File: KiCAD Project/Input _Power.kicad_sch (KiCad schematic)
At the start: 11 parts, among them J1 PJ-102B, Q1 BUK6D120-60PX

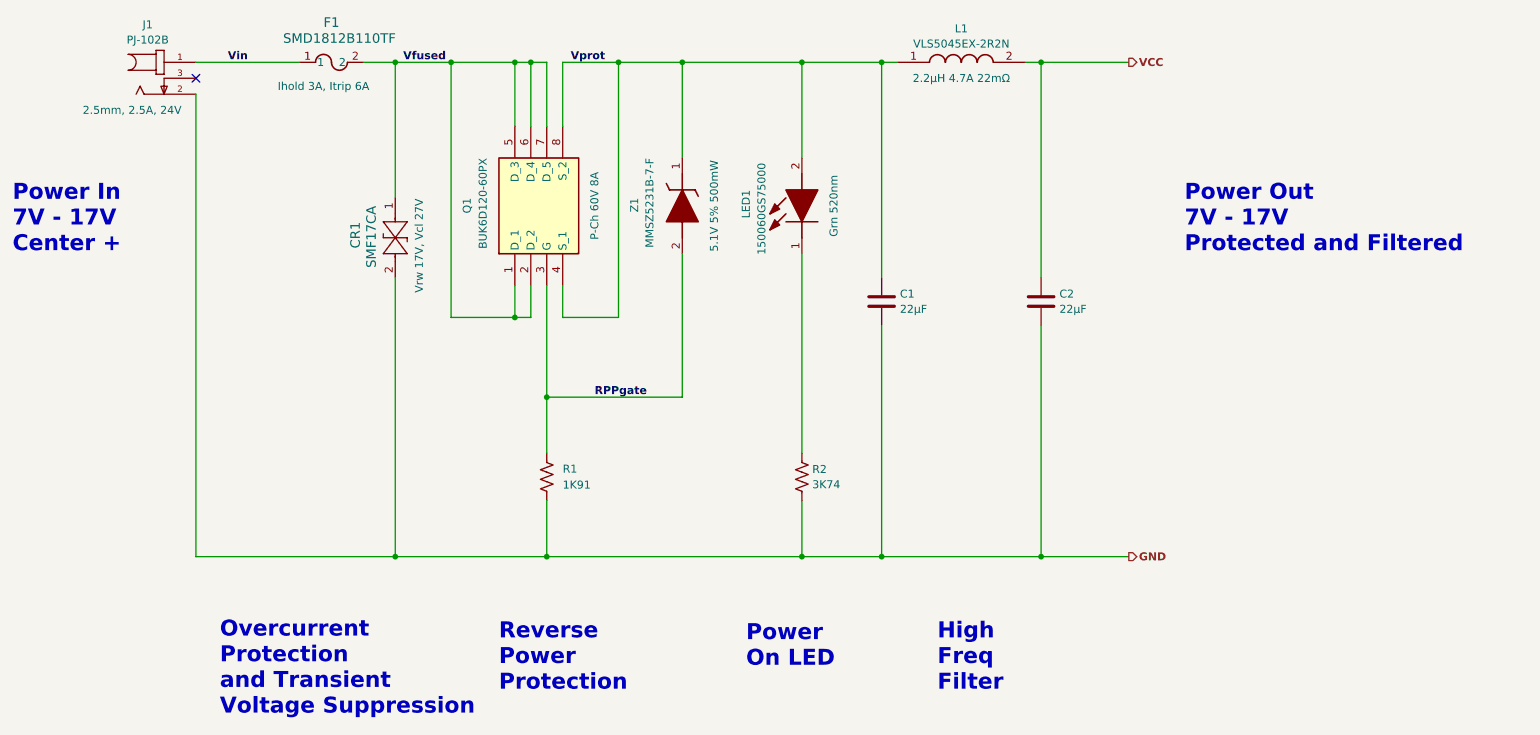
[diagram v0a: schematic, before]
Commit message: V1.0.0.0
Final version 1, sent for fabrication.
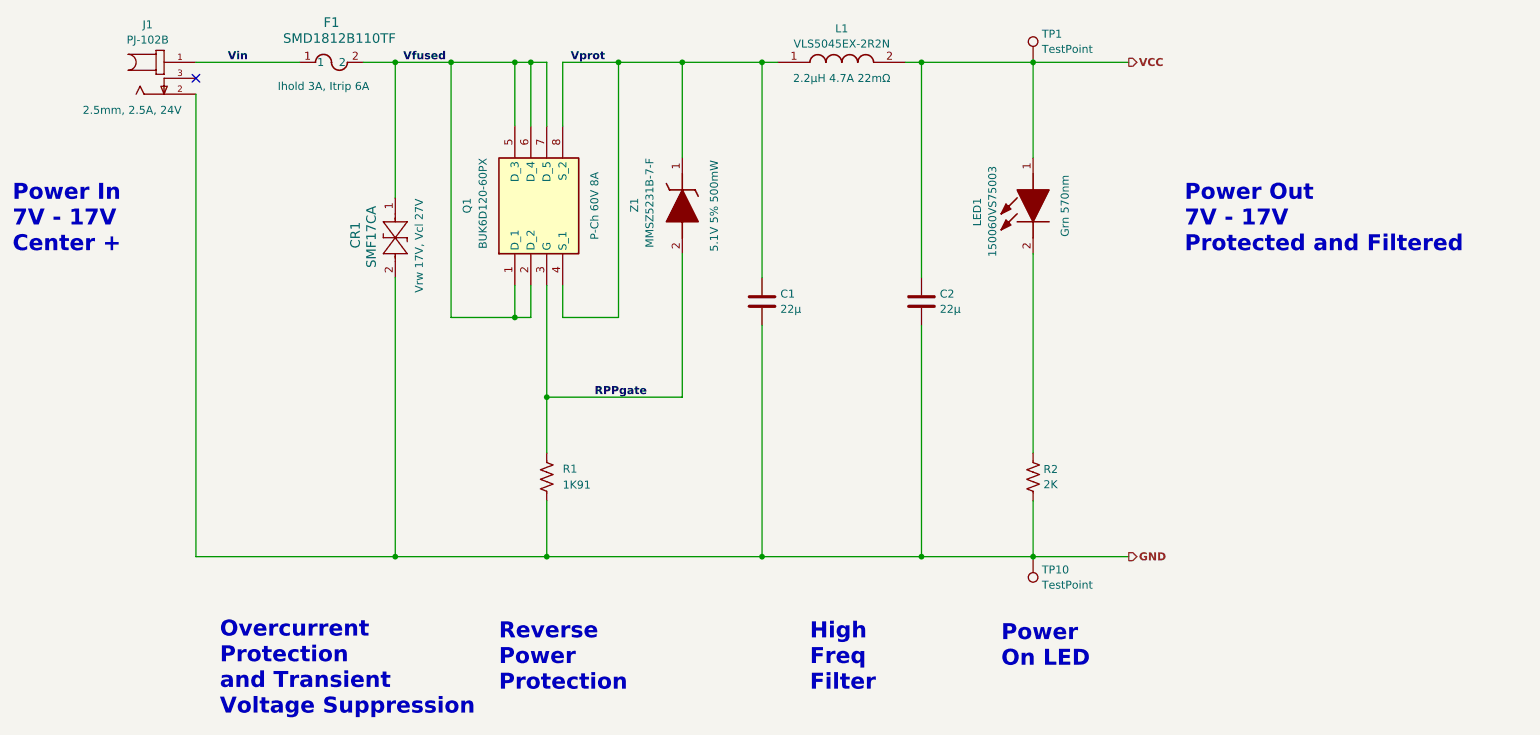
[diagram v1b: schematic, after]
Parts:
- removed LED1: 150060GS75000, LEDC1608X80N, symbol 1016:150060GS75000
- added LED1: 150060VS75003, 1016:LEDC1608X80N, symbol 1016:150060VS75003
- added TP1, TP10: TestPoint, TestPoint:TestPoint_THTPad_D1.0mm_Drill0.5mm, symbol Connector:TestPoint
- C1, C2: value 22µF -> 22µ; LCSC Part Number (none) -> C602037; Spec 22µF 25V -> 22µ 25V
- CR1: Manufacturer_Part_Number C3719828 -> SMF17CA
- Q1: footprint 1013v4:BUK6D12060PX -> 1016:BUK6D12060PX
- R2: value 3K74 -> 2K; footprint Resistor_SMD:R_0603_1608Metric -> Resistor_SMD:R_0805_2012Metric; Height 0.45 -> 0.5; LCSC Part Number C137728 -> C114572; Manufacturer_Part_Number RC0603FR-073K74L -> RC0805FR-072KL; Mouser Part Number 603-RC0603FR-073K74L -> 603-RC0805FR-072KL; Spec 3K74 100mW -> 2K 125mW
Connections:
- net GND: now also TP10.1
- net VCC: now also LED1.1 (A), TP1.1
- net at R2.1: now also LED1.2 (K)
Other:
- moved on the sheet: C1, C2, L1, R2
